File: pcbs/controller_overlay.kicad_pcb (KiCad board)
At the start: 2 copper layers, 19.2 x 58.5 mm, 2 parts

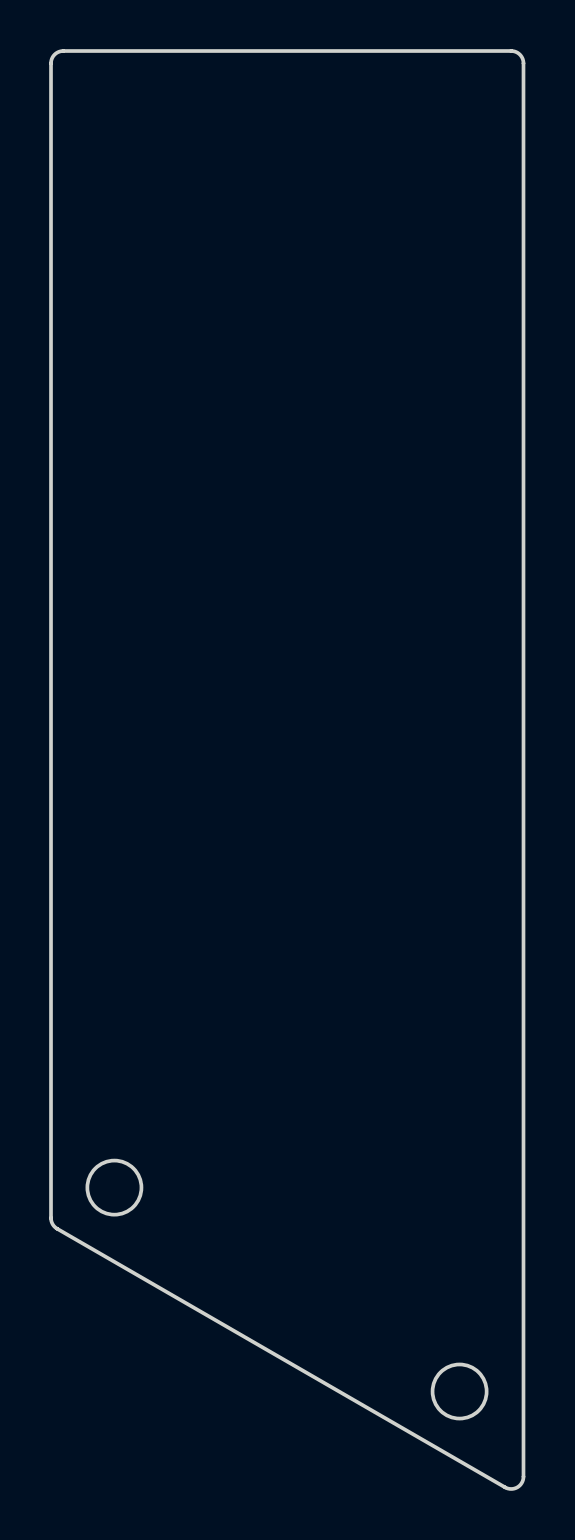
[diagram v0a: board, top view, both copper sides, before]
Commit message: Archive ordered wireless PCB and manufacturing files
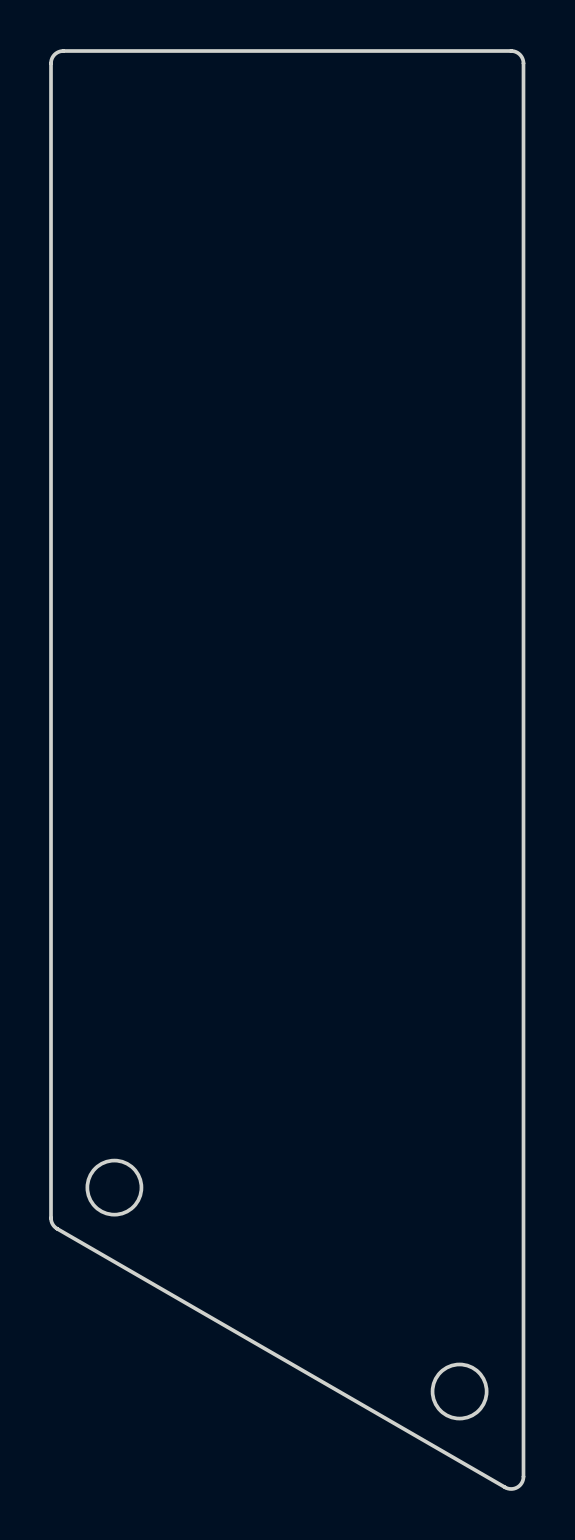
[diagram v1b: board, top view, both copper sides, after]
